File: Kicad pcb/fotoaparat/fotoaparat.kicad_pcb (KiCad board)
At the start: 2 copper layers, 104 x 114.5 mm, 36 parts, among them J1 Conn_02x01, J2 Conn_01x02_Socket, Q1 BC547, Q2 BC547, Q3 BC547, Q4 BC547, SW1 SW_Push_Dual, U1 TP4056, U10 VBsemi SI2312CDS-T1-GE3, U11 VBsemi SI2312CDS-T1-GE3, U12 VBsemi SI2312CDS-T1-GE3, U2 ov7670 fifo, U3 Stm32 Bluepill, U4 Lcd Display, U5 VBsemi SI2312CDS-T1-GE3, U6 Me6211c, U7 VBsemi SI2312CDS-T1-GE3, U8 Me6211c, U9 Me6211c

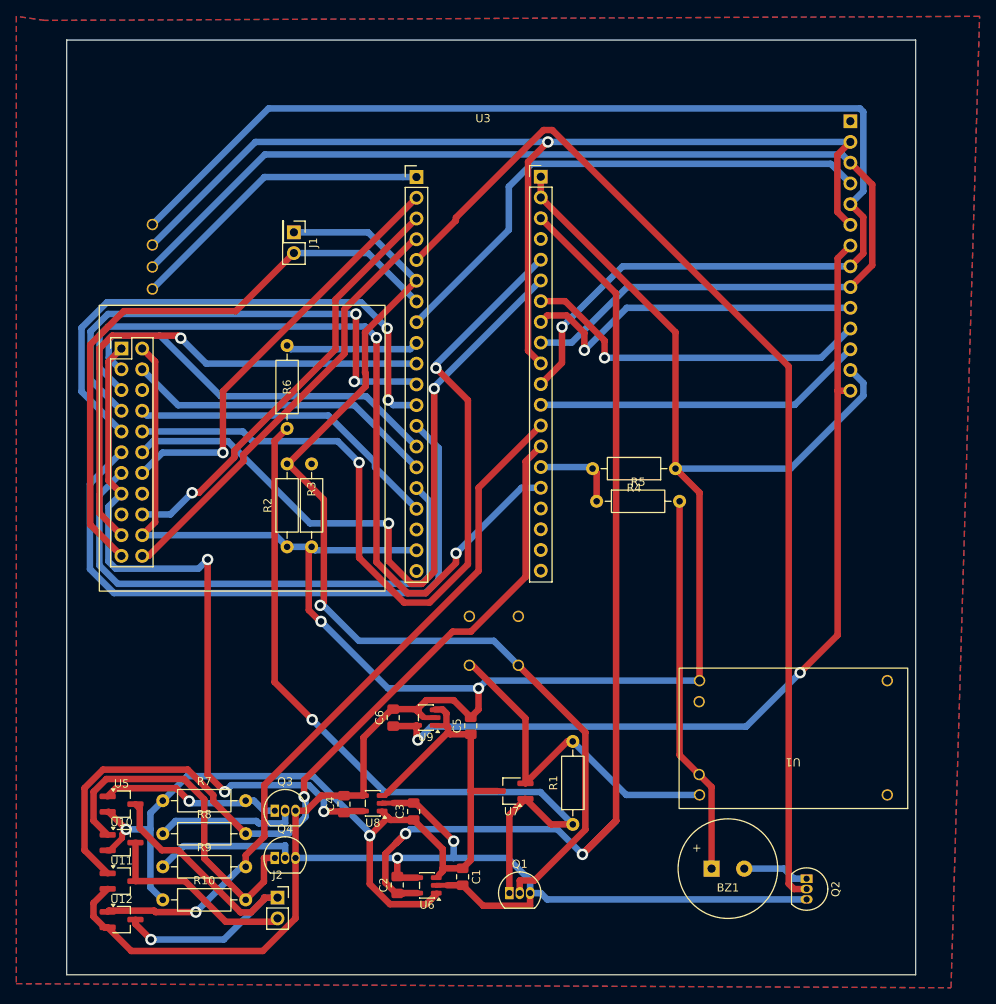
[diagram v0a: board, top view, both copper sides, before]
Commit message: Resistory
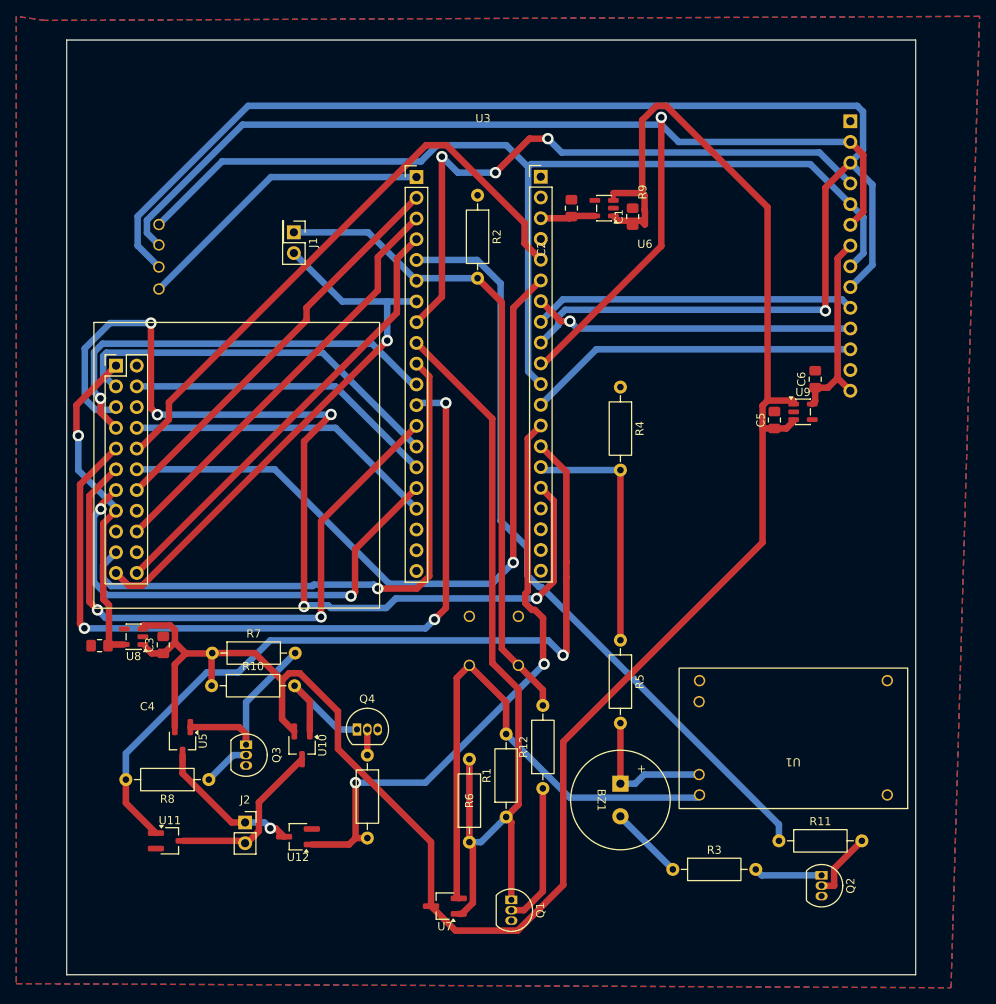
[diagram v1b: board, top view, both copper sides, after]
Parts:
- added R11: 1k, Resistor_THT:R_Axial_DIN0207_L6.3mm_D2.5mm_P10.16mm_Horizontal, F.Cu at (184.9, 139.0)
- added R12: 1k, Resistor_THT:R_Axial_DIN0207_L6.3mm_D2.5mm_P10.16mm_Horizontal, F.Cu at (156.0, 132.6)
- R2: value 100k -> 50k
- R3: value 10k -> 100
- R6: value 50k -> 1k
- moved U6 85.7 mm to (163.5, 61.5)
- moved C2 85.6 mm to (159.5, 61.5)
- moved C1 83.5 mm to (167.0, 62.5), turned to 90 degrees
- moved C6 66.3 mm to (189.4, 82.5)
- moved U9 59.5 mm to (187.9, 86.5), turned to 0 degrees
- moved R3 59.3 mm to (171.9, 142.5), turned to 0 degrees
- moved R6 55.4 mm to (147.0, 139.2)
- moved C5 52.8 mm to (184.4, 87.5)
- moved R2 49.0 mm to (148.0, 59.9), turned to -90 degrees
- moved C3 36.8 mm to (109.5, 115.0)
- moved U8 35.7 mm to (105.9, 114.0)
- moved C4 35.7 mm to (101.7, 115.1), turned to 180 degrees
- moved R9 28.6 mm to (134.5, 128.5), turned to -90 degrees
- moved BZ1 27.8 mm to (156.8, 134.0), turned to -90 degrees
- moved R10 26.9 mm to (115.4, 120.0)
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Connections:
- net Net-(U2-wr) renamed /wr
- Q1 pad 1: pow hold -> /pow hold
- Q1 pad 2: /tx + pow hold -> Net-(Q1-B)
- Q2 pad 1: Net-(BZ1--) -> Net-(Q2-C)
- Q2 pad 2: /zvuk -> Net-(Q2-B)
- R1 pad 1: pow hold -> /pow hold
- R3 pad 1: GND -> Net-(BZ1--)
- R3 pad 2: /tx -> Net-(Q2-C)
- R6 pad 1: pow hold -> /pow hold
- R6 pad 2: Net-(U3-pa12) -> /pow hold
- U3 pad 9: Net-(U3-pa12) -> /pow hold
- U6 pad 4: GND -> unconnected-(U6-NC-Pad4)
- U7 pad 1: pow hold -> /pow hold
- U8 pad 4: GND -> unconnected-(U8-NC-Pad4)
- U9 pad 4: GND -> unconnected-(U9-NC-Pad4)
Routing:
- net GND: track 401.6 -> 0.00 mm, vias 4 -> 0
- net +3.3V: track 148.3 -> 6.73 mm, vias 2 -> 0
- net +4V: track 127.4 -> 248.2 mm, vias 2 -> 0
- net /pow hold: track 0.00 -> 100.1 mm
- net pow hold: track 94.9 -> 0.00 mm, vias 1 -> 0
- net +3.3V lcd: track 111.4 -> 24.5 mm, vias 2 -> 0
- net +3.3V ov7670: track 90.0 -> 41.4 mm, vias 3 -> 1
- net /tx + pow hold: track 129.0 -> 80.7 mm, vias 1 -> 0
- net /zvuk: track 130.2 -> 94.1 mm
- net /mosi: track 149.8 -> 183.0 mm, vias 0 -> 1
- net /clk: track 160.5 -> 128.2 mm, vias 1 -> 0
- net /d5: track 67.4 -> 98.2 mm, vias 2 -> 3
- net +BATT: track 46.6 -> 17.5 mm
- net Net-(J2-Pin_1): track 46.2 -> 17.9 mm
- net /d4: track 101.6 -> 73.4 mm, vias 2 -> 0
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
